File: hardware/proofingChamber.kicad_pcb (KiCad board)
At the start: 2 copper layers, 40 x 67.5 mm, 15 parts, among them SW2 RotaryEncoder_Switch_MP, U1 ESP32-C3_SUPERMINI_TH, U2 DS18B20

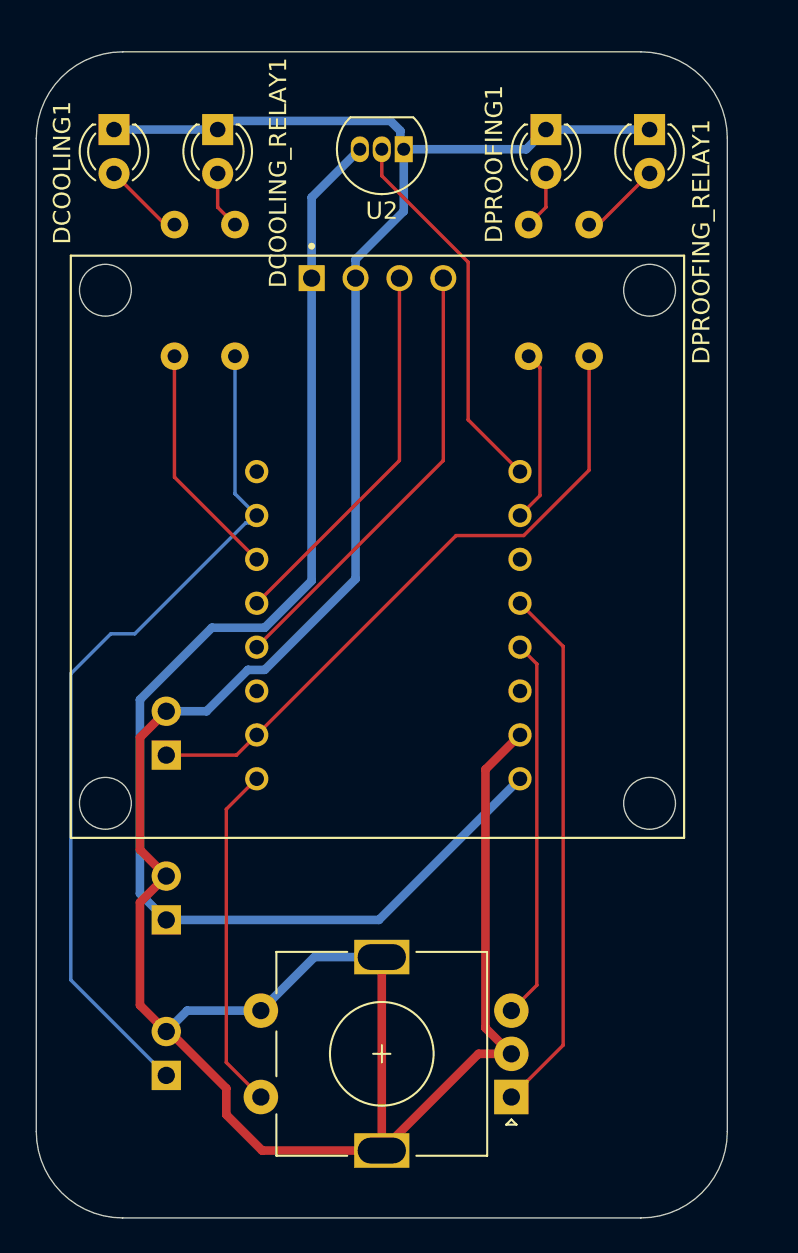
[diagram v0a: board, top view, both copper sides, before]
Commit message: Update PCB
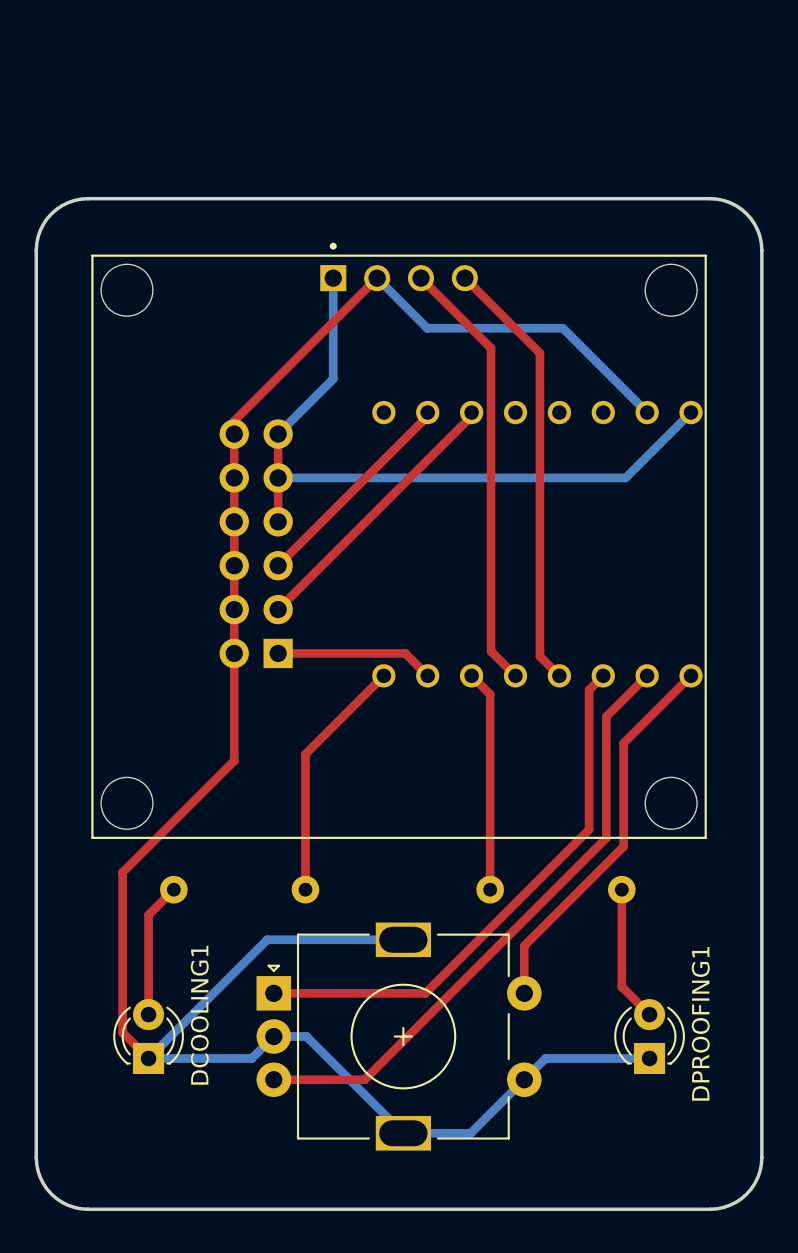
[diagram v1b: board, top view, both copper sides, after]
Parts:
- removed DCOOLING_RELAY1, DPROOFING_RELAY1: LED, LED_THT:LED_D3.0mm
- removed JCOOLING1, JPOWER, JPROOFING: Conn_01x02, Connector_PinSocket_2.54mm:PinSocket_1x02_P2.54mm_Vertical
- removed RCOOLING_RELAY_LED1, RPROOFING_RELAY_LED1: R, Resistor_THT:R_Axial_DIN0207_L6.3mm_D2.5mm_P7.62mm_Horizontal
- removed U2: DS18B20, Package_TO_SOT_THT:TO-92_Inline
- added J1: Conn_02x06_Odd_Even, Connector_PinSocket_2.54mm:PinSocket_2x06_P2.54mm_Horizontal, B.Cu at (231.5, 131.8)
- added REF**: OSHW-Logo2_9.8x8mm_SilkScreen, Symbol:OSHW-Logo2_9.8x8mm_SilkScreen, B.Cu at (238.8, 154.0)
- moved DPROOFING1 54.1 mm to (253.0, 155.3), turned to 90 degrees
- moved DCOOLING1 53.8 mm to (224.0, 155.3), turned to 90 degrees
- moved RPROOFING_LED1 38.9 mm to (251.4, 145.5), turned to 180 degrees
- moved RCOOLING_LED1 38.5 mm to (225.5, 145.5), turned to 0 degrees
- moved SW2 15.0 mm to (231.2, 151.5), turned to 0 degrees
- moved U1 8.46 mm to (245.5, 125.5), turned to 90 degrees
- moved DS1 1.25 mm to (238.5, 125.7)
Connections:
- U1 pad 0: /DS18B22_PIN -> unconnected-(U1-GPIO0-Pad0)
- U1 pad 1: /PROOFING_LED -> /PROOFING_RELAY
- U1 pad 10: /COOLING_LED -> /PROOFING_LED
- U1 pad 2: unconnected-(U1-GPIO2-Pad2) -> /COOLING_RELAY
- U1 pad 20: /COOLING_RELAY -> /DS18B22_PIN
- U1 pad 21: unconnected-(U1-GPIO21-Pad21) -> /COOLING_LED
- U1 pad 3: /ENCODER_A -> unconnected-(U1-GPIO3-Pad3)
- U1 pad 4: /ENCODER_B -> unconnected-(U1-GPIO4-Pad4)
- U1 pad 6: /PROOFING_RELAY -> /ENCODER_B
- U1 pad 7: unconnected-(U1-GPIO7-Pad7) -> /ENCODER_A
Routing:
- net GND: track 165.5 -> 122.2 mm
- net +5V: track 76.2 -> 40.9 mm
- net /COOLING_RELAY: track 49.8 -> 16.0 mm
- net /PROOFING_RELAY: track 37.5 -> 12.5 mm
- net /DS18B22_PIN: track 22.0 -> 8.57 mm
- net /ENCODER_B: track 22.1 -> 35.4 mm
- net Net-(DPROOFING_RELAY1-A): track 4.73 -> 0.00 mm
- net Net-(DPROOFING1-A): track 3.37 -> 7.90 mm
- net Net-(DCOOLING_RELAY1-A): track 3.37 -> 0.00 mm
- net Net-(DCOOLING1-A): track 4.73 -> 7.84 mm
- net /SCK: track 22.2 -> 25.3 mm
- net /PROOFING_LED: track 9.97 -> 12.8 mm
- net /ENCODER_BTN: track 20.0 -> 22.4 mm
- net /ENCODER_A: track 30.9 -> 31.4 mm
- net /SDA: track 25.8 -> 25.3 mm
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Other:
- board size 40 x 67.5 mm -> 42 x 58.5 mm
